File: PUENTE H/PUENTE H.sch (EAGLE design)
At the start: 20 parts, among them IC1 L293D, IC2 7805T

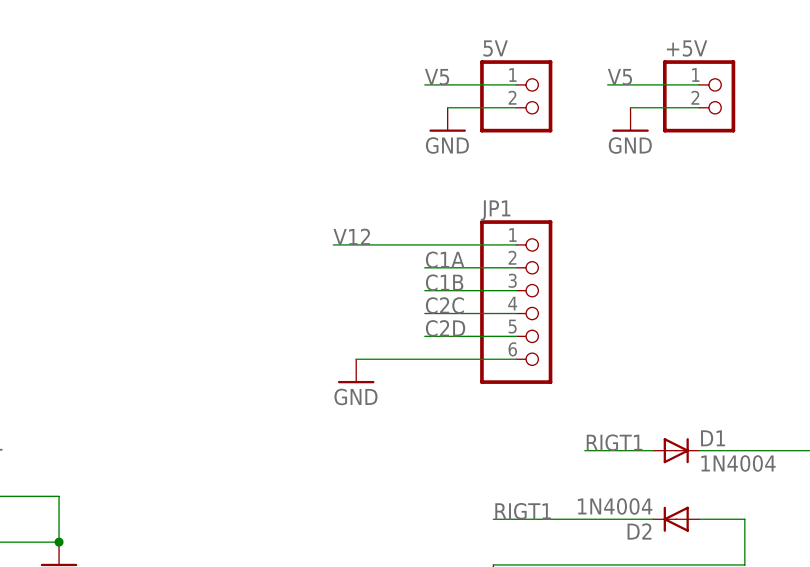
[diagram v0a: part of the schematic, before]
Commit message: archivos actualizados
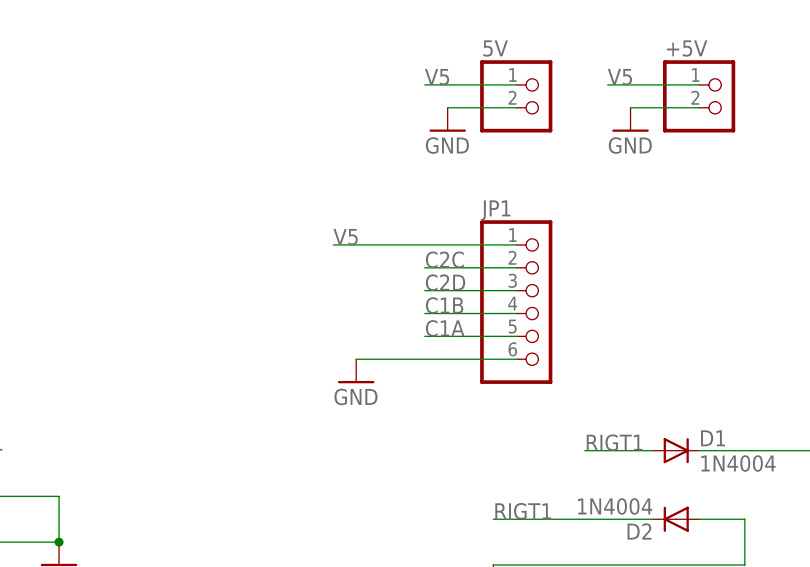
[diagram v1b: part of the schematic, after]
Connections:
- net C1A: now also JP1.5; no longer JP1.2
- net C1B: now also JP1.4; no longer JP1.3
- net C2C: now also JP1.2; no longer JP1.4
- net C2D: now also JP1.3; no longer JP1.5
- net V12: no longer JP1.1
- net V5: now also JP1.1
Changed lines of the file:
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@@
 </segment>
 <segment>
-<pinref part="JP1" gate="A" pin="2"/>
-<wire x1="203.2" y1="124.46" x2="193.04" y2="124.46" width="0.1524" layer="91"/>
-<label x="193.04" y="124.46" size="1.778" layer="95"/>
+<pinref part="JP1" gate="A" pin="5"/>
+<wire x1="203.2" y1="116.84" x2="193.04" y2="116.84" width="0.1524" layer="91"/>
+<label x="193.04" y="116.84" size="1.778" layer="95"/>
 </segment>
 </net>
@@
 </segment>
 <segment>
-<pinref part="JP1" gate="A" pin="3"/>
-<wire x1="203.2" y1="121.92" x2="193.04" y2="121.92" width="0.1524" layer="91"/>
-<label x="193.04" y="121.92" size="1.778" layer="95"/>
+<pinref part="JP1" gate="A" pin="4"/>
+<wire x1="203.2" y1="119.38" x2="193.04" y2="119.38" width="0.1524" layer="91"/>
+<label x="193.04" y="119.38" size="1.778" layer="95"/>
 </segment>
 </net>
@@
 </segment>
 <segment>
-<pinref part="JP1" gate="A" pin="5"/>
-<wire x1="203.2" y1="116.84" x2="193.04" y2="116.84" width="0.1524" layer="91"/>
-<label x="193.04" y="116.84" size="1.778" layer="95"/>
+<pinref part="JP1" gate="A" pin="3"/>
+<wire x1="203.2" y1="121.92" x2="193.04" y2="121.92" width="0.1524" layer="91"/>
+<label x="193.04" y="121.92" size="1.778" layer="95"/>
 </segment>
 </net>
@@
 </segment>
 <segment>
-<pinref part="JP1" gate="A" pin="4"/>
-<wire x1="203.2" y1="119.38" x2="193.04" y2="119.38" width="0.1524" layer="91"/>
-<label x="193.04" y="119.38" size="1.778" layer="95"/>
+<pinref part="JP1" gate="A" pin="2"/>
+<wire x1="203.2" y1="124.46" x2="193.04" y2="124.46" width="0.1524" layer="91"/>
+<label x="193.04" y="124.46" size="1.778" layer="95"/>
 </segment>
 </net>
@@
 </segment>
 <segment>
+<pinref part="+5V" gate="G$1" pin="1"/>
+<wire x1="223.52" y1="144.78" x2="213.36" y2="144.78" width="0.1524" layer="91"/>
+<label x="213.36" y="144.78" size="1.778" layer="95"/>
+</segment>
+<segment>
+<pinref part="JP1" gate="A" pin="1"/>
+<wire x1="203.2" y1="127" x2="182.88" y2="127" width="0.1524" layer="91"/>
+<label x="182.88" y="127" size="1.778" layer="95"/>
+</segment>
+<segment>
 <pinref part="5V" gate="G$1" pin="1"/>
 <wire x1="203.2" y1="144.78" x2="193.04" y2="144.78" width="0.1524" layer="91"/>
 <label x="193.04" y="144.78" size="1.778" layer="95"/>
-</segment>
-<segment>
-<pinref part="+5V" gate="G$1" pin="1"/>
-<wire x1="223.52" y1="144.78" x2="213.36" y2="144.78" width="0.1524" layer="91"/>
-<label x="213.36" y="144.78" size="1.778" layer="95"/>
 </segment>
 </net>
@@
 </segment>
 <segment>
-<pinref part="D6" gate="1" pin="C"/>
-<wire x1="25.4" y1="68.58" x2="12.7" y2="68.58" width="0.1524" layer="91"/>
-<label x="12.7" y="68.58" size="1.778" layer="95"/>
-</segment>
-<segment>
-<pinref part="D8" gate="1" pin="C"/>
-<wire x1="25.4" y1="91.44" x2="12.7" y2="91.44" width="0.1524" layer="91"/>
-<label x="12.7" y="91.44" size="1.778" layer="95"/>
-</segment>
-<segment>
 <pinref part="IC1" gate="G$1" pin="VCC2"/>
 <wire x1="104.14" y1="78.74" x2="99.06" y2="78.74" width="0.1524" layer="91"/>
 <label x="99.06" y="78.74" size="1.778" layer="95"/>
-</segment>
-<segment>
-<pinref part="JP1" gate="A" pin="1"/>
-<wire x1="203.2" y1="127" x2="182.88" y2="127" width="0.1524" layer="91"/>
-<label x="182.88" y="127" size="1.778" layer="95"/>
 </segment>
 <segment>
@@
 <label x="238.76" y="104.14" size="1.778" layer="95"/>
 </segment>
+<segment>
+<pinref part="D8" gate="1" pin="C"/>
+<wire x1="25.4" y1="91.44" x2="12.7" y2="91.44" width="0.1524" layer="91"/>
+<label x="12.7" y="91.44" size="1.778" layer="95"/>
+</segment>
+<segment>
+<pinref part="D6" gate="1" pin="C"/>
+<wire x1="25.4" y1="68.58" x2="12.7" y2="68.58" width="0.1524" layer="91"/>
+<label x="12.7" y="68.58" size="1.778" layer="95"/>
+</segment>
 </net>
